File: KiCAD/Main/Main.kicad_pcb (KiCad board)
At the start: 4 copper layers, 92 parts, among them J1 Micro_SD_Card_Det2, J2 Screw_Terminal_01x09, J3 Screw_Terminal_01x09, J4 USB_C_Receptacle_USB2.0_16P, J7 Conn_02x05_Top_Bottom_Mountin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, J8 Conn_Coaxial, Q1 AO3400A, Q2 AO3400A, Q3 AO3400A, Q4 2N7002, SW1 RESET, SW2 USER, U1 LM2596S-3.3, U11 BMP390L, U12 BMP390L, U13 BMP390L, U14 BMI270, U15 BMI270, U16 BMI270, U17 SHT4x, U2 TPS2121RUXR, U3 BMM350, U4 STM32H750VBTx, U5 MAX-M8Q, U7 ISM6HG256x, U9 BME280, Y2 SiT8008xx-2x-xxE (25MHz)

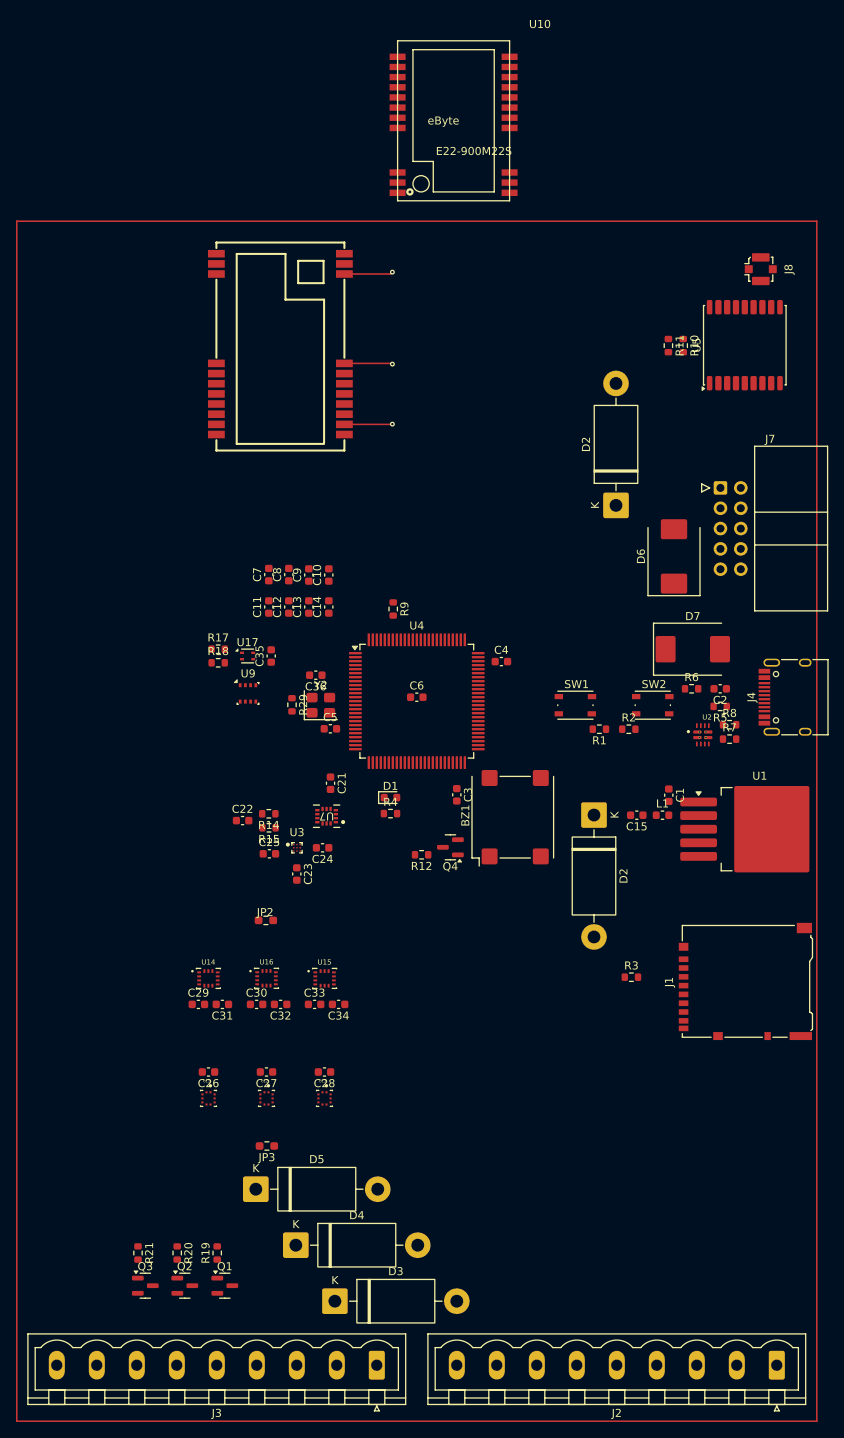
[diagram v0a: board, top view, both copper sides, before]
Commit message: 30%
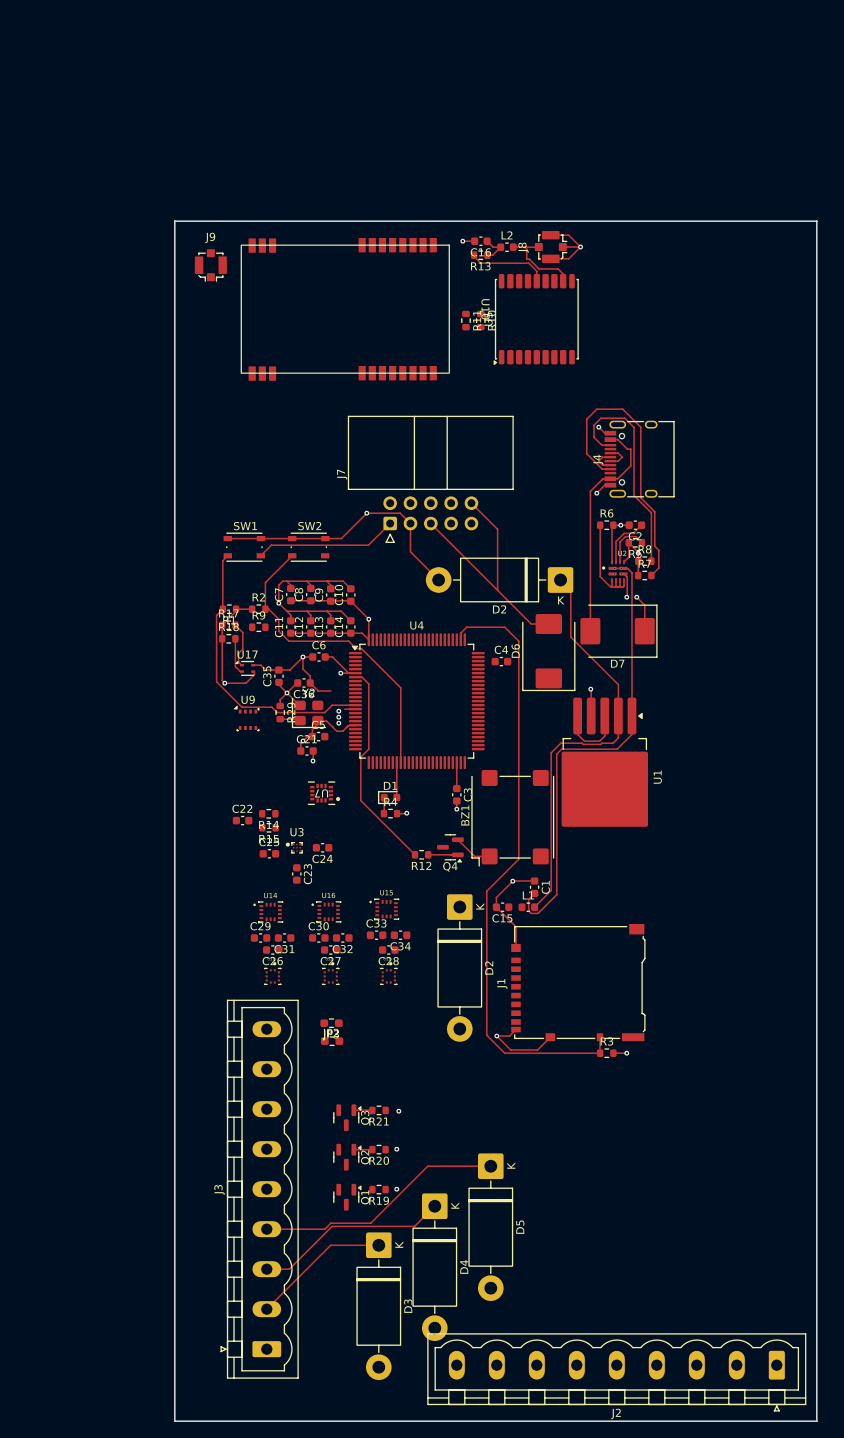
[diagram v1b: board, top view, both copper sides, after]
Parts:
- removed <Designator>?: E22-900T22S, E22-900T22S:E22-900T22S
- added C16: 10n, Capacitor_SMD:C_0603_1608Metric, F.Cu at (108.0, 42.5)
- added J9: Conn_Coaxial, Connector_Coaxial:U.FL_Molex_MCRF_73412-0110_Vertical, F.Cu at (74.3, 45.5)
- added L2: 47n, Inductor_SMD:L_0603_1608Metric, F.Cu at (111.3, 43.2)
- added R13: 10, Resistor_SMD:R_0603_1608Metric, F.Cu at (108.0, 44.2)
- U10: footprint E22-900M22S:E22-900M22S -> E22-900T22S:E22-900T22S
- moved R1 48.6 mm to (76.6, 88.5)
- moved R2 48.6 mm to (80.2, 88.5)
- moved SW2 47.3 mm to (86.5, 80.8)
- moved SW1 45.8 mm to (78.5, 80.8)
- moved J7 41.5 mm to (96.7, 77.8), turned to 90 degrees
- moved J4 35.4 mm to (128.2, 69.8)
- moved R21 35.0 mm to (95.3, 151.2), turned to 180 degrees
- moved Q3 32.7 mm to (91.2, 152.1), turned to -90 degrees
- moved D5 29.5 mm to (109.2, 158.1), turned to -90 degrees
- moved R20 28.3 mm to (95.3, 156.1), turned to 180 degrees
- moved U10 27.2 mm to (91.1, 51.0), turned to -90 degrees
- moved J8 26.4 mm to (116.8, 43.2), turned to -90 degrees
- moved U5 26.2 mm to (115.0, 52.2)
- moved Q2 25.8 mm to (91.2, 157.0), turned to -90 degrees
- moved R10 25.5 mm to (108.0, 52.4)
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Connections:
- C10 pad 1: Net-(U4-VDDA) -> +3V3
- C10 pad 2: +3V3 -> GND
- C11 pad 1: Net-(U4-VDDA) -> +3V3
- C11 pad 2: +3V3 -> GND
- C12 pad 1: Net-(U4-VDDA) -> +3V3
- C12 pad 2: +3V3 -> GND
- C13 pad 1: Net-(U4-VDDA) -> +3V3
- C13 pad 2: +3V3 -> GND
- C14 pad 1: Net-(U4-VDDA) -> +3V3
- C14 pad 2: +3V3 -> GND
- C6 pad 1: +3V3 -> GND
- C7 pad 1: Net-(U4-VDDA) -> +3V3
- C7 pad 2: +3V3 -> GND
- C8 pad 1: Net-(U4-VDDA) -> +3V3
- C8 pad 2: +3V3 -> GND
- C9 pad 1: Net-(U4-VDDA) -> +3V3
- C9 pad 2: +3V3 -> GND
- U10 pad 1: /RF/NOTE: Using built-in coaxial antenna port -> Net-(J9-In)
- U4 pad 100: Net-(U4-VDDA) -> +3V3
- U4 pad 11: Net-(U4-VDDA) -> +3V3
- U4 pad 21: Net-(U4-VDDA) -> +3V3
- U4 pad 27: Net-(U4-VDDA) -> +3V3
- U4 pad 50: Net-(U4-VDDA) -> +3V3
- U4 pad 75: Net-(U4-VDDA) -> +3V3
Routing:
- net GND: track 6.01 -> 154.1 mm, vias 1 -> 14
- net /Microcontroller/SD_Det: track 0.00 -> 77.2 mm
- net +3V3: track 0.00 -> 60.7 mm, vias 0 -> 7
- net Net-(U1-VIN): track 0.00 -> 59.7 mm
- net /~{RESET}: track 0.00 -> 53.5 mm
- net Net-(D2-K): track 0.00 -> 52.2 mm
- net /Microcontroller/USER_BTN: track 0.00 -> 39.3 mm
- net Net-(J4-CC1): track 0.00 -> 36.1 mm
- net Net-(D6-A): track 0.00 -> 32.2 mm
- net Net-(D5-K): track 0.00 -> 31.3 mm
- net Net-(D7-A): track 0.00 -> 29.0 mm
- net Net-(J4-CC2): track 0.00 -> 27.4 mm
- net Net-(U4-PC13): track 0.00 -> 26.6 mm
- net Net-(D4-K): track 0.00 -> 24.3 mm
- net Net-(D3-K): track 0.00 -> 17.3 mm
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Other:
- board outline added: 80.2 x 150 mm
